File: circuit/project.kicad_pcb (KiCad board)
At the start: 4 copper layers, 95 x 50 mm, 109 parts, among them J1 VIN, J2 ANT, J3 Conn_01x03, J4 VOUT, J5 Conn_01x03, M1 Debugger, Q1 S8050, Q2 ME85P03, SW1 SW_DIP_x01, SW2 SW_DIP_x01, U1 HX9193, U10 π131M31, U11 ATGM336H, U12 XPT2046TS, U2 REF3030, U3 TPS54540, U4 SY8303, U5 MM32F3277G9P, U6 ADIS16470AMLZ, U7 B0505S-1WR3, U8 HX9193, U9 π131M31, Y1 8MHz

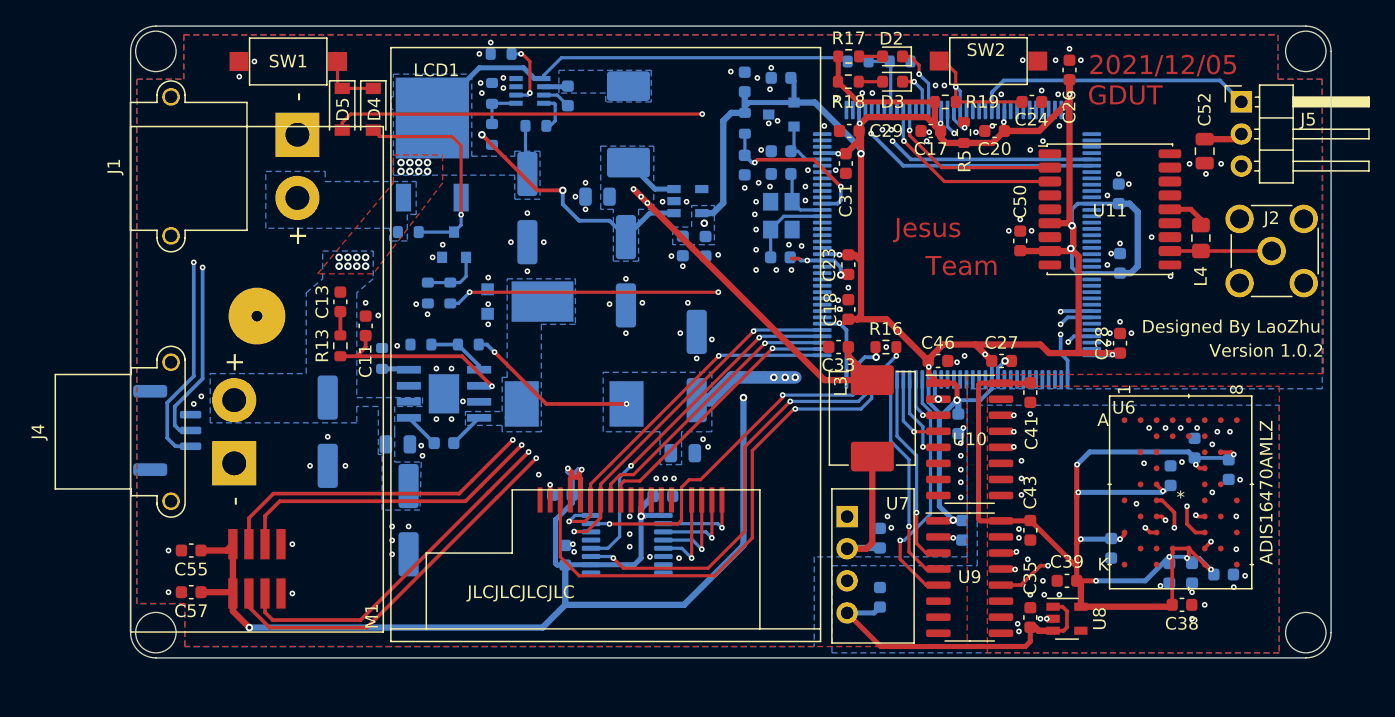
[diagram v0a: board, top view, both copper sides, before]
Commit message: Update circuit project to KiCAD 6.0.0 version
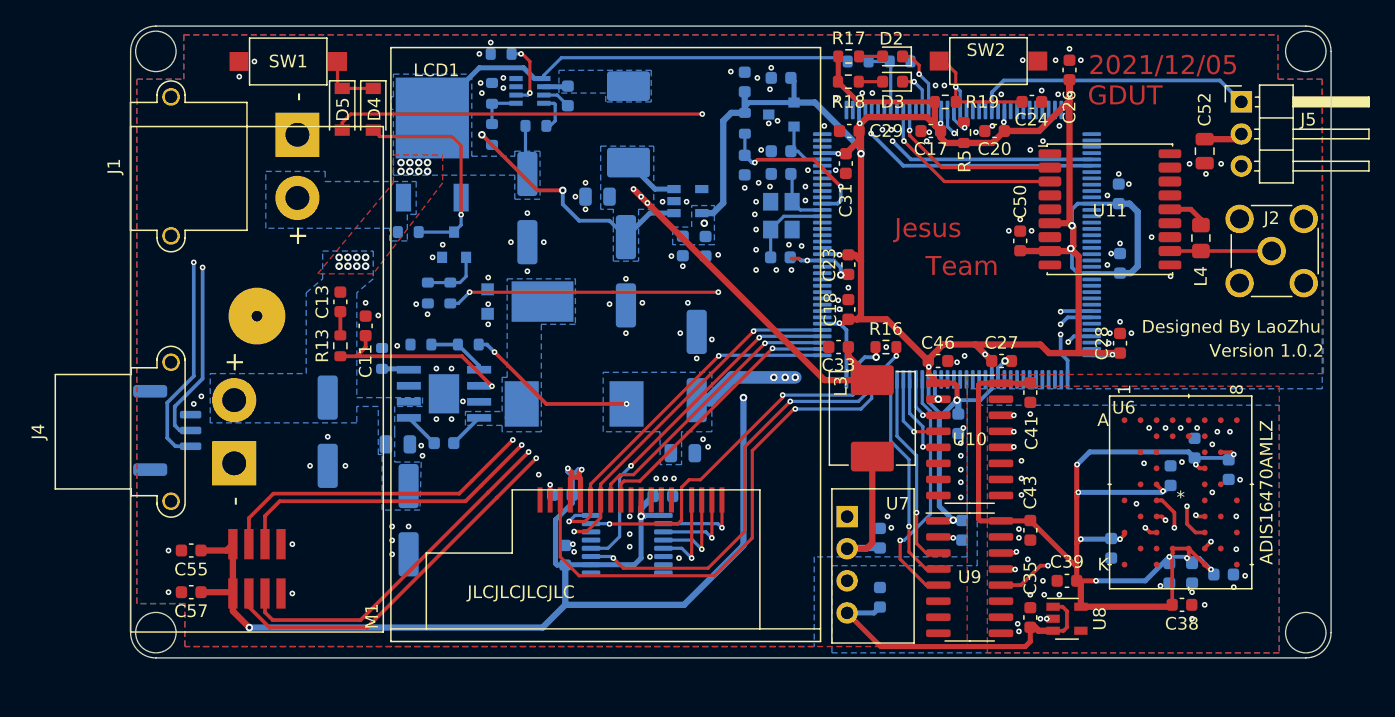
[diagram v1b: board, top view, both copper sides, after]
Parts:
- C1, C11, C12, C13, C17, C18, C19, C2, C20, C21, C22, C23, C24, C25, C26, C27, C28, C29, C30, C31, C32, C33, C34, C35, C36, C37, C38, C39, C4, C40, C41, C42, C43, C44, C45, C46, C47, C48, C49, C50, C53, C54, C55, C56, C57, C58, C6, C9: footprint Capacitor_SMD:C_0603_1608Metric -> MM32_Library:C_0603_1608Metric
- C10, C14, C51, C52: footprint Capacitor_SMD:C_0805_2012Metric -> MM32_Library:C_0805_2012Metric
- C15, C16, C5, C7, C8: footprint Capacitor_SMD:CP_Elec_6.3x7.7 -> MM32_Library:CP_Elec_6.3x7.7
- D1: footprint Package_TO_SOT_SMD:TO-277B -> MM32_Library:TO-277B
- D2, D3: footprint LED_SMD:LED_0603_1608Metric -> MM32_Library:LED_0603_1608Metric
- D4, D5: footprint Diode_SMD:D_SOD-123 -> MM32_Library:D_SOD-123
- J1: footprint Connector_AMASS:AMASS_XT30PW-M_1x02_P2.50mm_Horizontal -> MM32_Library:AMASS_XT30PW-M_1x02_P2.50mm_Horizontal
- J2: footprint Connector_Coaxial:SMA_Molex_73251-2200_Horizontal -> MM32_Library:SMA_Molex_73251-2200_Horizontal
- J3: footprint Connector_JST:JST_GH_SM03B-GHS-TB_1x03-1MP_P1.25mm_Horizontal -> MM32_Library:JST_GH_SM03B-GHS-TB_1x03-1MP_P1.25mm_Horizontal
- J4: footprint Connector_AMASS:AMASS_XT30PW-F_1x02_P2.50mm_Horizontal -> MM32_Library:AMASS_XT30PW-F_1x02_P2.50mm_Horizontal
- J5: footprint Connector_PinHeader_2.54mm:PinHeader_1x03_P2.54mm_Horizontal -> MM32_Library:PinHeader_1x03_P2.54mm_Horizontal
- L1: footprint Inductor_SMD:L_10.4x10.4_H4.8 -> MM32_Library:L_10.4x10.4_H4.8
- L2, L3: footprint Inductor_SMD:L_Abracon_ASPI-0630LR -> MM32_Library:L_Abracon_ASPI-0630LR
- L4: footprint Inductor_SMD:L_0805_2012Metric_Pad1.15x1.40mm_HandSolder -> MM32_Library:L_0805_2012Metric_Pad1.15x1.40mm_HandSolder
- LCD1: footprint Display:TFT-LCD1.8inch -> MM32_Library:TFT-LCD1.8inch
- M1: footprint Connector:Gernic_Debugger -> MM32_Library:Gernic_Debugger
- Q1, U2: footprint Package_TO_SOT_SMD:SOT-23 -> MM32_Library:SOT-23
- Q2: footprint Package_TO_SOT_SMD:TO-252-2 -> MM32_Library:TO-252-2
- R1, R10, R11, R12, R13, R14, R15, R16, R17, R18, R19, R2, R20, R3, R5, R6, R7, R8, R9: footprint Resistor_SMD:R_0603_1608Metric -> MM32_Library:R_0603_1608Metric
- SW1, SW2: footprint Button_Switch_SMD:SW_SPST_CK_RS282G05A3 -> MM32_Library:SW_SPST_CK_RS282G05A3
- U1, U8: footprint Package_TO_SOT_SMD:SOT-23-5 -> MM32_Library:SOT-23-5
- U10, U9: footprint Package_SO:SOIC-16_3.9x9.9mm_P1.27mm -> MM32_Library:SOIC-16_3.9x9.9mm_P1.27mm
- U11: footprint RF_GPS:ublox_MAX -> MM32_Library:ublox_MAX
- U12: footprint Package_SO:TSSOP-16_4.4x5mm_P0.65mm -> MM32_Library:TSSOP-16_4.4x5mm_P0.65mm
- U3: footprint Package_SO:TI_SO-PowerPAD-8 -> MM32_Library:TI_SO-PowerPAD-8
- U4: footprint Package_TO_SOT_SMD:SOT-23-8 -> MM32_Library:SOT-23-8
- U5: footprint Package_QFP:LQFP-144_20x20mm_P0.5mm -> MM32_Library:LQFP-144_20x20mm_P0.5mm
- U6: footprint Sensor_Motion:ADIS16470AMLZ -> MM32_Library:ADIS16470AMLZ
- U7: footprint Package_SIP:SIP-4_B0505S_1WR3 -> MM32_Library:SIP-4_B0505S_1WR3
- Y1: footprint Crystal:Crystal_SMD_3225-4Pin_3.2x2.5mm -> MM32_Library:Crystal_SMD_3225-4Pin_3.2x2.5mm
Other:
- net class Default removed

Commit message: Update circuit and ADIS16470 footprint reference datasheet.
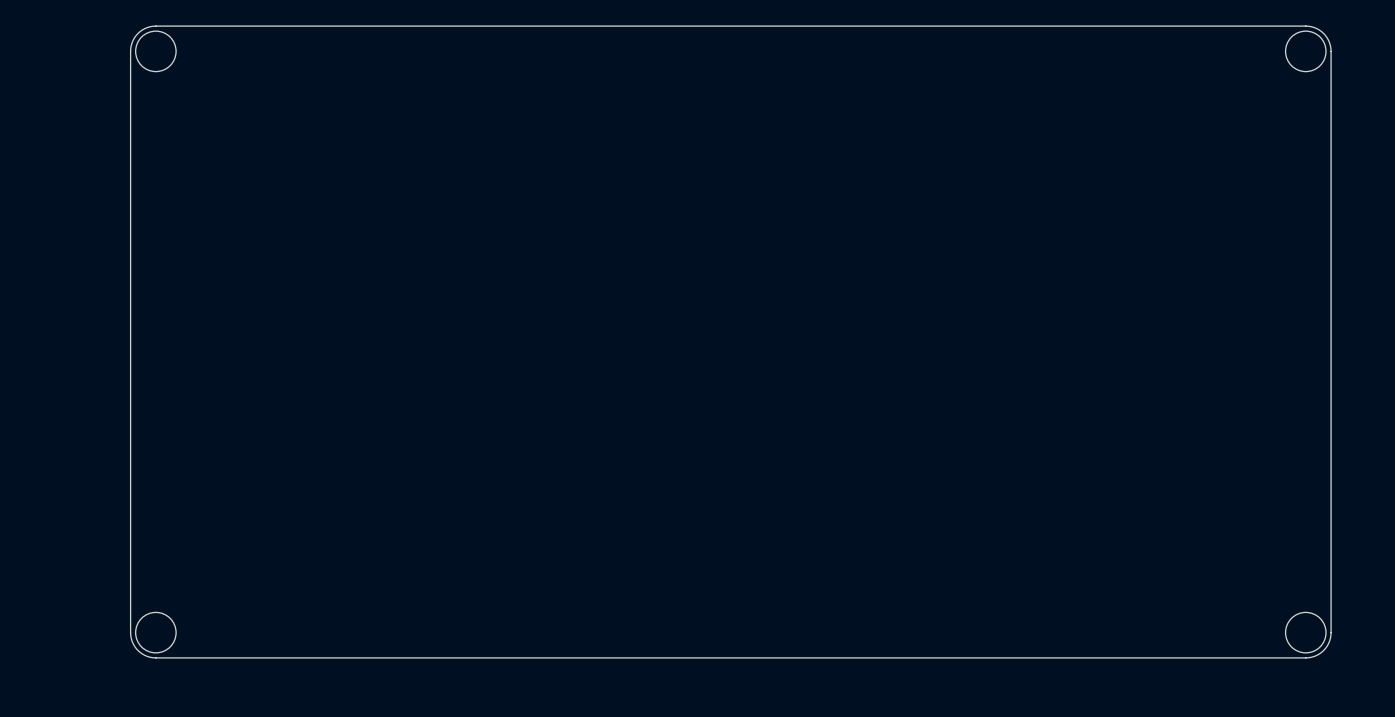
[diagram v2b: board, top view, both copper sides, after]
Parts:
- removed C1, C43: 22uF, MM32_Library:C_0603_1608Metric
- removed C10: 10uF, MM32_Library:C_0805_2012Metric
- removed C11: 32pF, MM32_Library:C_0603_1608Metric
- removed C12: 10nF, MM32_Library:C_0603_1608Metric
- removed C13: 620pF, MM32_Library:C_0603_1608Metric
- removed C14, C51, C52: 22uF, MM32_Library:C_0805_2012Metric
- removed C15, C16, C5, C7, C8: 100uF, MM32_Library:CP_Elec_6.3x7.7
- removed C17, C18, C2, C20, C21, C22, C23, C24, C26, C27, C28, C29, C30, C31, C32, C36, C37, C38, C39, C4, C40, C41, C42, C44, C45, C46, C47, C48, C49, C53, C54, C55, C56, C57, C58, C6, C9: 100nF, MM32_Library:C_0603_1608Metric
- removed C19, C25: 18pF, MM32_Library:C_0603_1608Metric
- removed C33, C34, C35, C50: 10uF, MM32_Library:C_0603_1608Metric
- removed D1: SVM1550UB, MM32_Library:TO-277B
- removed D2, D3: LED, MM32_Library:LED_0603_1608Metric
- removed D4, D5: 1N4007, MM32_Library:D_SOD-123
- removed J1: VIN, MM32_Library:AMASS_XT30PW-M_1x02_P2.50mm_Horizontal
- removed J2: ANT, MM32_Library:SMA_Molex_73251-2200_Horizontal
- removed J3: Conn_01x03, MM32_Library:JST_GH_SM03B-GHS-TB_1x03-1MP_P1.25mm_Horizontal
- removed J4: VOUT, MM32_Library:AMASS_XT30PW-F_1x02_P2.50mm_Horizontal
- removed J5: Conn_01x03, MM32_Library:PinHeader_1x03_P2.54mm_Horizontal
- removed L1: 3.3uH, MM32_Library:L_10.4x10.4_H4.8
- removed L2: 4.7uH, MM32_Library:L_Abracon_ASPI-0630LR
- removed L3: 6.8uH, MM32_Library:L_Abracon_ASPI-0630LR
- removed L4: 47nH, MM32_Library:L_0805_2012Metric_Pad1.15x1.40mm_HandSolder
- removed LCD1: 1.8inch-TFT-LCD, MM32_Library:TFT-LCD1.8inch
- removed M1: Debugger, MM32_Library:Gernic_Debugger
- removed Q1: S8050, MM32_Library:SOT-23
- removed Q2: ME85P03, MM32_Library:TO-252-2
- removed R1, R12, R8: 100kR, MM32_Library:R_0603_1608Metric
- removed R10: 86.6kR, MM32_Library:R_0603_1608Metric
- removed R11: 47kR, MM32_Library:R_0603_1608Metric
- removed R13: 23.7kR, MM32_Library:R_0603_1608Metric
- removed R14: 82kR, MM32_Library:R_0603_1608Metric
- removed R15, R16, R19, R2, R20, R5, R6: 10kR, MM32_Library:R_0603_1608Metric
- removed R17, R18, R7: 1kR, MM32_Library:R_0603_1608Metric
- removed R3: 100R, MM32_Library:R_0603_1608Metric
- removed R9: 13.6kR, MM32_Library:R_0603_1608Metric
- removed SW1, SW2: SW_DIP_x01, MM32_Library:SW_SPST_CK_RS282G05A3
- removed U1, U8: HX9193, MM32_Library:SOT-23-5
- removed U10, U9: π131M31, MM32_Library:SOIC-16_3.9x9.9mm_P1.27mm
- removed U11: ATGM336H, MM32_Library:ublox_MAX
- removed U12: XPT2046TS, MM32_Library:TSSOP-16_4.4x5mm_P0.65mm
- removed U2: REF3030, MM32_Library:SOT-23
- removed U3: TPS54540, MM32_Library:TI_SO-PowerPAD-8
- removed U4: SY8303, MM32_Library:SOT-23-8
- removed U5: MM32F3277G9P, MM32_Library:LQFP-144_20x20mm_P0.5mm
- removed U6: ADIS16470AMLZ, MM32_Library:ADIS16470AMLZ
- removed U7: B0505S-1WR3, MM32_Library:SIP-4_B0505S_1WR3
- removed Y1: 8MHz, MM32_Library:Crystal_SMD_3225-4Pin_3.2x2.5mm
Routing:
- net +3V3: track 318.0 -> 0.00 mm, vias 21 -> 0
- net +3.3VA: track 94.9 -> 0.00 mm, vias 11 -> 0
- net /Connector/MOTOR_TX: track 93.2 -> 0.00 mm, vias 2 -> 0
- net /Connector/MOTOR_RX: track 89.9 -> 0.00 mm, vias 2 -> 0
- net /Connector/SWDIO: track 78.5 -> 0.00 mm, vias 2 -> 0
- net /Connector/SWDCLK: track 78.4 -> 0.00 mm, vias 2 -> 0
- net /Connector/DEBUG_RX: track 75.6 -> 0.00 mm, vias 2 -> 0
- net /Connector/DEBUG_TX: track 74.6 -> 0.00 mm, vias 2 -> 0
- net +7.5V: track 70.2 -> 0.00 mm, vias 5 -> 0
- net +5V: track 54.1 -> 0.00 mm, vias 5 -> 0
- net /MCU/PF14: track 52.9 -> 0.00 mm, vias 2 -> 0
- net /MCU/PF13: track 51.9 -> 0.00 mm, vias 3 -> 0
- net /Connector/LCD_CS: track 41.1 -> 0.00 mm, vias 1 -> 0
- net +15V: track 40.9 -> 0.00 mm, vias 16 -> 0
- net /MCU/PE0: track 32.9 -> 0.00 mm, vias 2 -> 0
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- removed copper zone on B.Cu, net +15V
- removed copper zone on F.Cu, net +15V
- removed copper zone on B.Cu, net +3V3
- removed copper zone on B.Cu, net +5V
- removed copper zone on B.Cu, net +7.5V
- removed copper zone on B.Cu, net EP
- removed copper zone on F.Cu, net EP
- removed copper zone on In1.Cu, net EP
- removed copper zone on In2.Cu, net EP
- removed copper zone on B.Cu, net GNDA
- removed copper zone on F.Cu, net GNDA
- removed copper zone on In1.Cu, net GNDA
- removed copper zone on In2.Cu, net GNDA
- removed copper zone on B.Cu, net Net-(C12-Pad1)
- removed copper zone on B.Cu, net Net-(C9-Pad1)
- removed copper zone on B.Cu, net VDD
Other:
- board text removed: "2021/12/05"
- board text removed: "Designed By LaoZhu"
- board text removed: "GDUT"
- board text removed: "JLCJLCJLCJLC"
- board text removed: "Jesus"
- board text removed: "Team"
- board text removed: "Version 1.0.2"

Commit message: Complete the PCB drawing and DRC check.
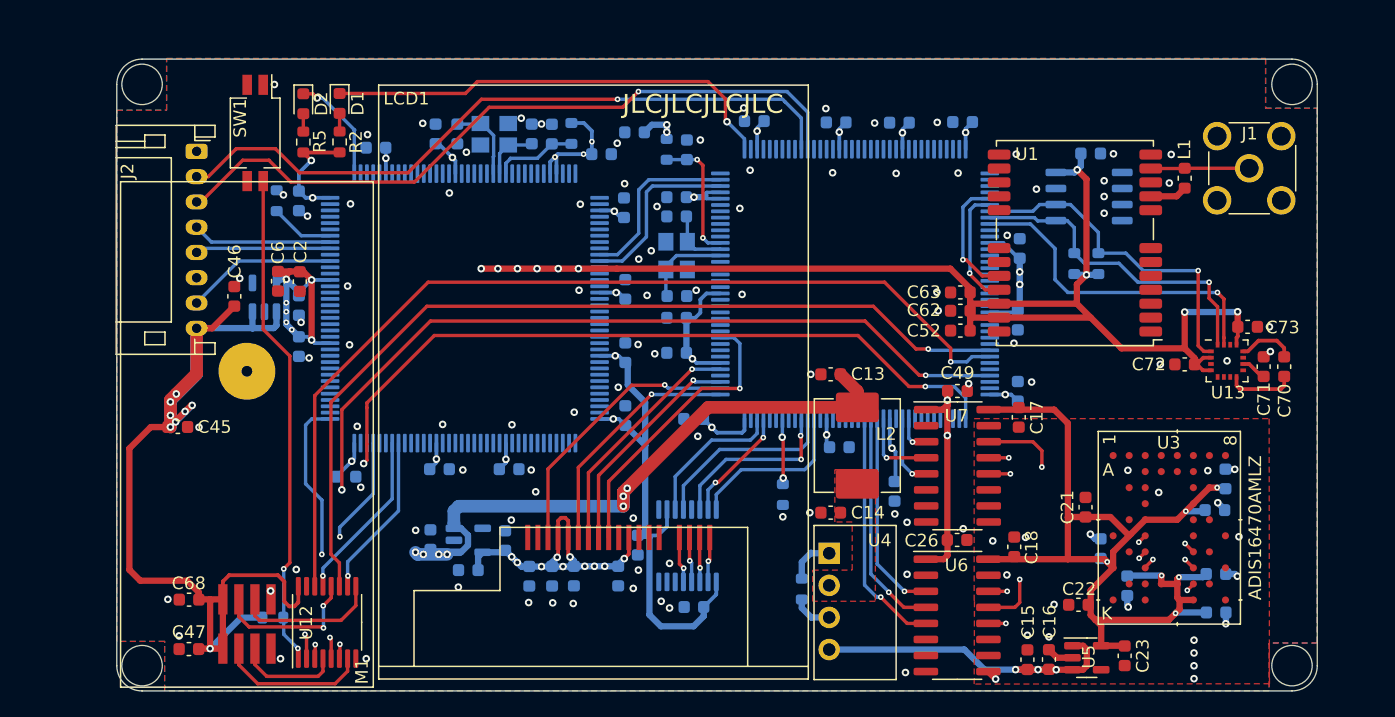
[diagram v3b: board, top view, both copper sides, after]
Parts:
- added C1: 100nF, Capacitor_SMD:C_0603_1608Metric, B.Cu at (144.2, 100.8)
- added C10: 100nF, Capacitor_SMD:C_0603_1608Metric, B.Cu at (149.6, 101.1)
- added C11: 100nF, Capacitor_SMD:C_0603_1608Metric, B.Cu at (170.8, 77.6)
- added C12: 100nF, Capacitor_SMD:C_0603_1608Metric, B.Cu at (175.2, 93.3)
- added C13: 10uF, Capacitor_SMD:C_0603_1608Metric, F.Cu at (160.4, 97.6)
- added C14: 10uF, Capacitor_SMD:C_0603_1608Metric, F.Cu at (160.4, 108.5)
- added C15: 10uF, Capacitor_SMD:C_0603_1608Metric, F.Cu at (176.0, 120.1)
- added C16: 100nF, Capacitor_SMD:C_0603_1608Metric, F.Cu at (177.7, 120.1)
- added C17: 100nF, Capacitor_SMD:C_0603_1608Metric, F.Cu at (175.3, 101.0)
- added C18: 100nF, Capacitor_SMD:C_0603_1608Metric, F.Cu at (174.9, 111.2)
- added C19: 100nF, Capacitor_SMD:C_0603_1608Metric, B.Cu at (181.8, 111.3)
- added C2: 100nF, Capacitor_SMD:C_0603_1608Metric, F.Cu at (118.4, 90.2)
- added C20: 100nF, Capacitor_SMD:C_0603_1608Metric, B.Cu at (183.9, 114.3)
- added C21: 100nF, Capacitor_SMD:C_0603_1608Metric, F.Cu at (180.6, 108.1)
- added C22: 100nF, Capacitor_SMD:C_0603_1608Metric, F.Cu at (180.0, 115.8)
- added C23: 22uF, Capacitor_SMD:C_0603_1608Metric, F.Cu at (183.7, 119.8)
- added C24: 100nF, Capacitor_SMD:C_0603_1608Metric, B.Cu at (190.9, 116.4)
- added C25: 100nF, Capacitor_SMD:C_0603_1608Metric, B.Cu at (190.8, 108.3)
- added C26: 100nF, Capacitor_SMD:C_0603_1608Metric, F.Cu at (170.4, 110.7)
- added C27: 100nF, Capacitor_SMD:C_0603_1608Metric, B.Cu at (148.2, 83.5)
- added C28: 100nF, Capacitor_SMD:C_0603_1608Metric, B.Cu at (191.6, 105.8)
- added C29: 100nF, Capacitor_SMD:C_0603_1608Metric, B.Cu at (190.9, 113.4)
- added C3: 100nF, Capacitor_SMD:C_0603_1608Metric, B.Cu at (124.4, 79.6)
- added C30: 100nF, Capacitor_SMD:C_0603_1608Metric, B.Cu at (161.1, 103.3)
- added C31: 100nF, Capacitor_SMD:C_0603_1608Metric, B.Cu at (143.6, 113.5)
- added C32: 18pF, Capacitor_SMD:C_0603_1608Metric, B.Cu at (148.2, 85.1)
- added C33: 100nF, Capacitor_SMD:C_0603_1608Metric, B.Cu at (144.9, 78.4)
- added C34: 100nF, Capacitor_SMD:C_0603_1608Metric, B.Cu at (138.4, 113.5)
- added C35: 100nF, Capacitor_SMD:C_0603_1608Metric, B.Cu at (140.1, 113.5)
- added C36: 100nF, Capacitor_SMD:C_0603_1608Metric, B.Cu at (154.4, 77.5)
- added C37: 18pF, Capacitor_SMD:C_0603_1608Metric, B.Cu at (148.2, 91.4)
- added C38: 100nF, Capacitor_SMD:C_0603_1608Metric, B.Cu at (148.2, 93.1)
- added C39: 100nF, Capacitor_SMD:C_0603_1608Metric, B.Cu at (136.6, 113.5)
- added C4: 100nF, Capacitor_SMD:C_0603_1608Metric, B.Cu at (135.0, 105.1)
- added C40: 100nF, Capacitor_SMD:C_0603_1608Metric, B.Cu at (134.6, 110.7)
- added C41: 100nF, Capacitor_SMD:C_0603_1608Metric, B.Cu at (160.8, 77.6)
- added C42: 100nF, Capacitor_SMD:C_0603_1608Metric, B.Cu at (149.0, 79.8)
- added C43: 100nF, Capacitor_SMD:C_0603_1608Metric, B.Cu at (131.7, 113.1)
- added C44: 100nF, Capacitor_SMD:C_0603_1608Metric, B.Cu at (148.2, 95.9)
- added C45: 10uF, Capacitor_SMD:C_0603_1608Metric, F.Cu at (108.7, 101.7)
- added C46: 10uF, Capacitor_SMD:C_0603_1608Metric, F.Cu at (113.2, 91.4)
- added C47: 100nF, Capacitor_SMD:C_0603_1608Metric, F.Cu at (109.6, 119.3)
- added C48: 22uF, Capacitor_SMD:C_0603_1608Metric, B.Cu at (165.8, 77.6)
- added C49: 100nF, Capacitor_SMD:C_0603_1608Metric, F.Cu at (170.4, 98.9)
- added C5: 100nF, Capacitor_SMD:C_0603_1608Metric, B.Cu at (129.4, 105.1)
- added C50: 22uF, Capacitor_SMD:C_0603_1608Metric, B.Cu at (149.6, 116.0)
- added C51: 100nF, Capacitor_SMD:C_0603_1608Metric, B.Cu at (145.1, 111.1)
- added C52: 100nF, Capacitor_SMD:C_0603_1608Metric, F.Cu at (170.7, 94.1)
- added C53: 100nF, Capacitor_SMD:C_0603_1608Metric, B.Cu at (144.2, 90.8)
- added C54: 18pF, Capacitor_SMD:C_0603_1608Metric, B.Cu at (136.7, 78.5)
- added C55: 100nF, Capacitor_SMD:C_0603_1608Metric, B.Cu at (129.1, 78.5)
- added C56: 100nF, Capacitor_SMD:C_0603_1608Metric, B.Cu at (118.3, 83.8)
- added C57: 100nF, Capacitor_SMD:C_0603_1608Metric, B.Cu at (118.3, 92.1)
- added C58: 100nF, Capacitor_SMD:C_0603_1608Metric, B.Cu at (122.0, 105.7)
- added C59: 18pF, Capacitor_SMD:C_0603_1608Metric, B.Cu at (130.9, 78.5)
- added C6: 100nF, Capacitor_SMD:C_0603_1608Metric, F.Cu at (116.7, 90.2)
- added C60: 100nF, Capacitor_SMD:C_0603_1608Metric, B.Cu at (144.2, 95.8)
- added C61: 100nF, Capacitor_SMD:C_0603_1608Metric, B.Cu at (142.3, 80.1)
- added C62: 100nF, Capacitor_SMD:C_0603_1608Metric, F.Cu at (170.7, 92.5)
- added C63: 100nF, Capacitor_SMD:C_0603_1608Metric, F.Cu at (170.7, 91.1)
- added C64: 100nF, Capacitor_SMD:C_0603_1608Metric, B.Cu at (138.3, 78.5)
- added C65: 100nF, Capacitor_SMD:C_0603_1608Metric, B.Cu at (118.3, 95.4)
- added C66: 100nF, Capacitor_SMD:C_0603_1608Metric, B.Cu at (144.0, 84.4)
- added C67: 10uF, Capacitor_SMD:C_0603_1608Metric, B.Cu at (128.7, 110.6)
- added C68: 100nF, Capacitor_SMD:C_0603_1608Metric, F.Cu at (109.6, 115.4)
- added C69: 100nF, Capacitor_SMD:C_0603_1608Metric, B.Cu at (181.0, 80.1)
- added C7: 100nF, Capacitor_SMD:C_0603_1608Metric, B.Cu at (165.5, 106.8)
- added C70: 220nF, Capacitor_SMD:C_0603_1608Metric, F.Cu at (196.3, 96.9)
- added C71: 4.7uF, Capacitor_SMD:C_0603_1608Metric, F.Cu at (194.7, 96.9)
- added C72: 100nF, Capacitor_SMD:C_0603_1608Metric, F.Cu at (188.4, 96.8)
- added C73: 100nF, Capacitor_SMD:C_0603_1608Metric, F.Cu at (193.4, 93.8)
- added C8: 100nF, Capacitor_SMD:C_0603_1608Metric, B.Cu at (175.4, 87.6)
- added C9: 100nF, Capacitor_SMD:C_0603_1608Metric, B.Cu at (175.2, 98.9)
- added D1: LED, LED_SMD:LED_0603_1608Metric, F.Cu at (121.5, 76.1)
- added D2: LED, LED_SMD:LED_0603_1608Metric, F.Cu at (118.7, 76.1)
- added J1: ANT, Connector_Coaxial:SMA_Molex_73251-2200_Horizontal, F.Cu at (193.5, 81.3)
- added J2: Conn_01x08, Connector_JST:JST_PH_S8B-PH-K_1x08_P2.00mm_Horizontal, F.Cu at (110.2, 79.9)
- added L1: 39nH, Inductor_SMD:L_0603_1608Metric, F.Cu at (188.4, 82.0)
- added L2: 6.8uH, Inductor_SMD:L_Abracon_ASPI-0630LR, F.Cu at (162.5, 103.2)
- added LCD1: 1.8inch-TFT-LCD, MM32_Library:TFT-LCD1.8inch, F.Cu at (124.6, 121.9)
- added M1: Debugger, MM32_Library:Gernic_Debugger, F.Cu at (124.2, 122.3)
- added R1: 10kR, Resistor_SMD:R_0603_1608Metric, B.Cu at (156.6, 107.1)
- added R10: 2.2kR, Resistor_SMD:R_0603_1608Metric, B.Cu at (181.6, 88.8)
- added R2: 1kR, Resistor_SMD:R_0603_1608Metric, F.Cu at (121.5, 79.2)
- added R3: 10kR, Resistor_SMD:R_0603_1608Metric, B.Cu at (147.4, 79.8)
- added R4: 10kR, Resistor_SMD:R_0603_1608Metric, B.Cu at (116.6, 83.8)
- added R5: 1kR, Resistor_SMD:R_0603_1608Metric, F.Cu at (118.7, 79.2)
- added R6: 10kR, Resistor_SMD:R_0603_1608Metric, B.Cu at (139.9, 78.5)
- added R7: 10kR, Resistor_SMD:R_0603_1608Metric, B.Cu at (116.3, 116.8)
- added R8: 10kR, Resistor_SMD:R_0603_1608Metric, B.Cu at (158.1, 114.6)
- added R9: 2.2kR, Resistor_SMD:R_0603_1608Metric, B.Cu at (179.7, 88.8)
- added SW1: SW_DIP_x02, Button_Switch_SMD:SW_DIP_SPSTx02_Slide_Copal_CHS-02B_W7.62mm_P1.27mm, F.Cu at (114.9, 78.5)
- added U1: TAU1201, RF_GPS:ublox_NEO, F.Cu at (179.7, 87.2)
- added U10: HX9193, Package_TO_SOT_SMD:SOT-23-5, B.Cu at (115.6, 91.5)
- added U11: MM32F3277G9P, Package_QFP:LQFP-144_20x20mm_P0.5mm, B.Cu at (131.5, 92.3)
- added U12: CH440R, Package_SO:TSSOP-16_4.4x5mm_P0.65mm, F.Cu at (120.5, 117.2)
- added U13: HMC5883L, MM32_Library:QFN-16_3x3_Pitch0.5mm, F.Cu at (191.8, 96.5)
- added U14: AT24C02, Package_SO:SOP-8_3.9x4.9mm_P1.27mm, B.Cu at (180.8, 83.5)
- added U2: XPT2046TS, Package_SO:TSSOP-16_4.4x5mm_P0.65mm, B.Cu at (149.1, 111.1)
- added U3: ADIS16470AMLZ, MM32_Library:ADIS16470AMLZ, F.Cu at (187.2, 109.7)
- added U4: B0505S-1WR3, MM32_Library:SIP-4_B0505S_1WR3, F.Cu at (160.3, 111.7)
- added U5: HX9193, Package_TO_SOT_SMD:SOT-23-5, F.Cu at (180.7, 120.0)
- added U6: π131M31, Package_SO:SOIC-16_3.9x9.9mm_P1.27mm, F.Cu at (170.4, 116.6)
- added U7: π131M31, Package_SO:SOIC-16_3.9x9.9mm_P1.27mm, F.Cu at (170.4, 104.8)
- added U8: MM32F3277G9P, Package_QFP:LQFP-144_20x20mm_P0.5mm, B.Cu at (162.3, 90.4)
- added U9: HX9193, Package_TO_SOT_SMD:SOT-23-5, B.Cu at (131.7, 110.7)
- added Y1: 8MHz, Crystal:Crystal_SMD_3225-4Pin_3.2x2.5mm, B.Cu at (148.2, 88.2)
- added Y2: 8MHz, Crystal:Crystal_SMD_3225-4Pin_3.2x2.5mm, B.Cu at (133.8, 78.6)
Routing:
- net +3.3VP: track 0.00 -> 199.5 mm, vias 0 -> 31
- net +5V: track 0.00 -> 159.8 mm, vias 0 -> 15
- net +3.3VA: track 0.00 -> 92.8 mm, vias 0 -> 26
- net +3.3VADC: track 0.00 -> 76.9 mm, vias 0 -> 6
- net /Debugger/SWDCLK1: track 0.00 -> 76.4 mm, vias 0 -> 3
- net /Debugger/SWDIO1: track 0.00 -> 76.1 mm, vias 0 -> 3
- net /Debugger/DBG_TX1: track 0.00 -> 75.6 mm, vias 0 -> 1
- net /Debugger/DBG_RX1: track 0.00 -> 71.6 mm, vias 0 -> 1
- net /Power/PWR_TX: track 0.00 -> 57.0 mm, vias 0 -> 1
- net /Power/PWR_RX: track 0.00 -> 55.1 mm, vias 0 -> 1
- net /Debugger/SEL: track 0.00 -> 39.3 mm, vias 0 -> 2
- net /Process_MCU/LED1: track 0.00 -> 36.1 mm, vias 0 -> 1
- net /Compass&Storage/IIC_SCL: track 0.00 -> 27.0 mm, vias 0 -> 1
- net +5VA: track 0.00 -> 26.9 mm, vias 0 -> 3
- net /Compass&Storage/COMPASS_RDY: track 0.00 -> 26.1 mm, vias 0 -> 1
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- added copper zone on In1.Cu, net +3.3VA
- added copper zone on In1.Cu, net +3.3VP
- added copper zone on B.Cu, net GND
- added copper zone on F.Cu, net GND
- added copper zone on In1.Cu, net GND
- added copper zone on In2.Cu, net GND
- added copper zone on F.Cu, net GNDA
- added copper zone on In1.Cu, net GNDA
- added copper zone on In2.Cu, net GNDA
- added copper zone on F.Cu, net Net-(C14-Pad1)
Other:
- board text added: "0"
- board text added: "0 mm"
- board text added: "0.0127 mm"
- board text added: "0.0175 mm"
- board text added: "0.02"
- board text added: "0.035 mm"
- board text added: "0.1000 mm / 0.2000 mm"
- board text added: "0.2 mm"
- board text added: "0.2000 mm"
- board text added: "1"
- board text added: "1.065 mm"
- board text added: "1.5954 mm"
- board text added: "2022/01/18"
- board text added: "3.5"
- board text added: "4"
- board text added: "4.6"
- board text added: "95.1000 mm x 50.1000 mm"
- board text added: "B.Cu"
- board text added: "B.Mask"
- board text added: "B.Paste"
- board text added: "B.Silkscreen"
- board text added: "BOARD CHARACTERISTICS"
- board text added: "Black"
- board text added: "Bottom Silk Screen"
- board text added: "Bottom Solder Mask"
- board text added: "Bottom Solder Paste"
- board text added: "Designed By"
- board text added: "Epsilon R（相对介电常数）"
- board text added: "F.Cu"
- board text added: "F.Mask"
- board text added: "F.Paste"
- board text added: "F.Silkscreen"
- board text added: "FR4"
- board text added: "GDUT"
- board text added: "HAL SnPb"
- board text added: "In1.Cu"
- board text added: "In2.Cu"
- board text added: "JLC7628"
- board text added: "JLCJLCJLCJLC"
- board text added: "Jesus"
- board text added: "LaoZhu"
- board text added: "Loss Tangent（损耗切线）"
- board text added: "MM32 Control Board"
- board text added: "Mask"
- board text added: "Not specified"
- board text added: "Team"
- board text added: "Top Silk Screen"
- board text added: "Top Solder Mask"
- board text added: "Top Solder Paste"
- board text added: "Version 1.2.2"
- board text added: "White"
- board text added: "copper"
- board text added: "prepreg"
- board text added: "否"
- board text added: "孔最小直径："
- board text added: "层名称"
- board text added: "最小布线/间距："
- board text added: "材料"
- board text added: "板子整体尺寸："
- board text added: "电介质层 1"
- board text added: "电介质层 2"
- board text added: "电介质层 3"
- board text added: "电路板厚度："
- board text added: "电镀板边："
- board text added: "类型"
- board text added: "粗细 (mm)"
- board text added: "边缘卡连接器："
- board text added: "邮票孔："
- board text added: "铜层数量："
- board text added: "铜表面处理（镀铜）："
- board text added: "阻抗控制"
- board text added: "颜色"
